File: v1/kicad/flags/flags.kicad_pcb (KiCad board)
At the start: 2 copper layers, 156.5 x 107.5 mm, 13 parts, among them J1 LNCPU_FLAGS_Connector, U1 74LS32, U10 74LS08, U11 74HC173, U12 74LS244, U2 74LS08, U3 74LS32, U4 74AHC04, U5 74LS32, U6 74LS157, U7 74LS157, U8 LNCPU Type B Connector, U9 74HC74

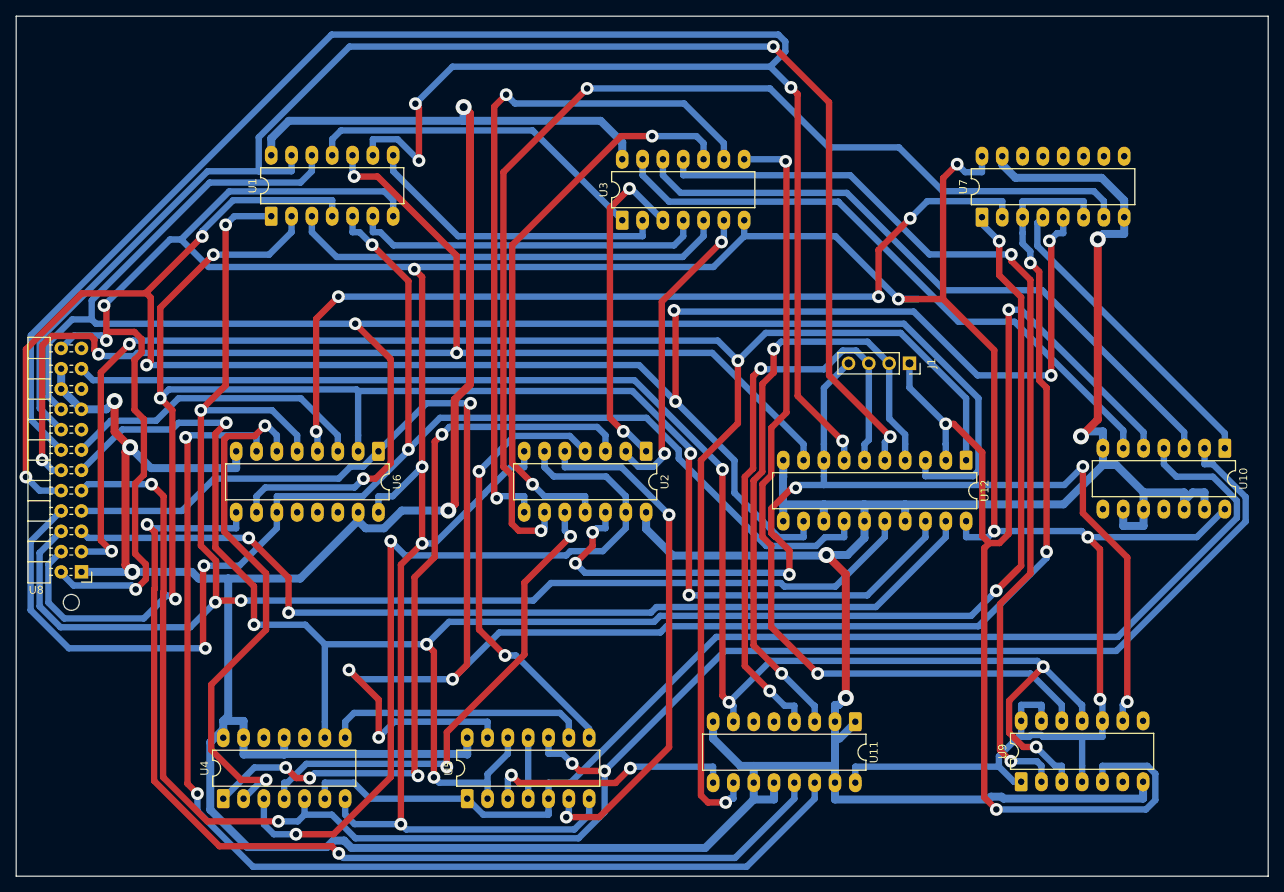
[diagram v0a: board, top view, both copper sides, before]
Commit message: partial on kicad flags
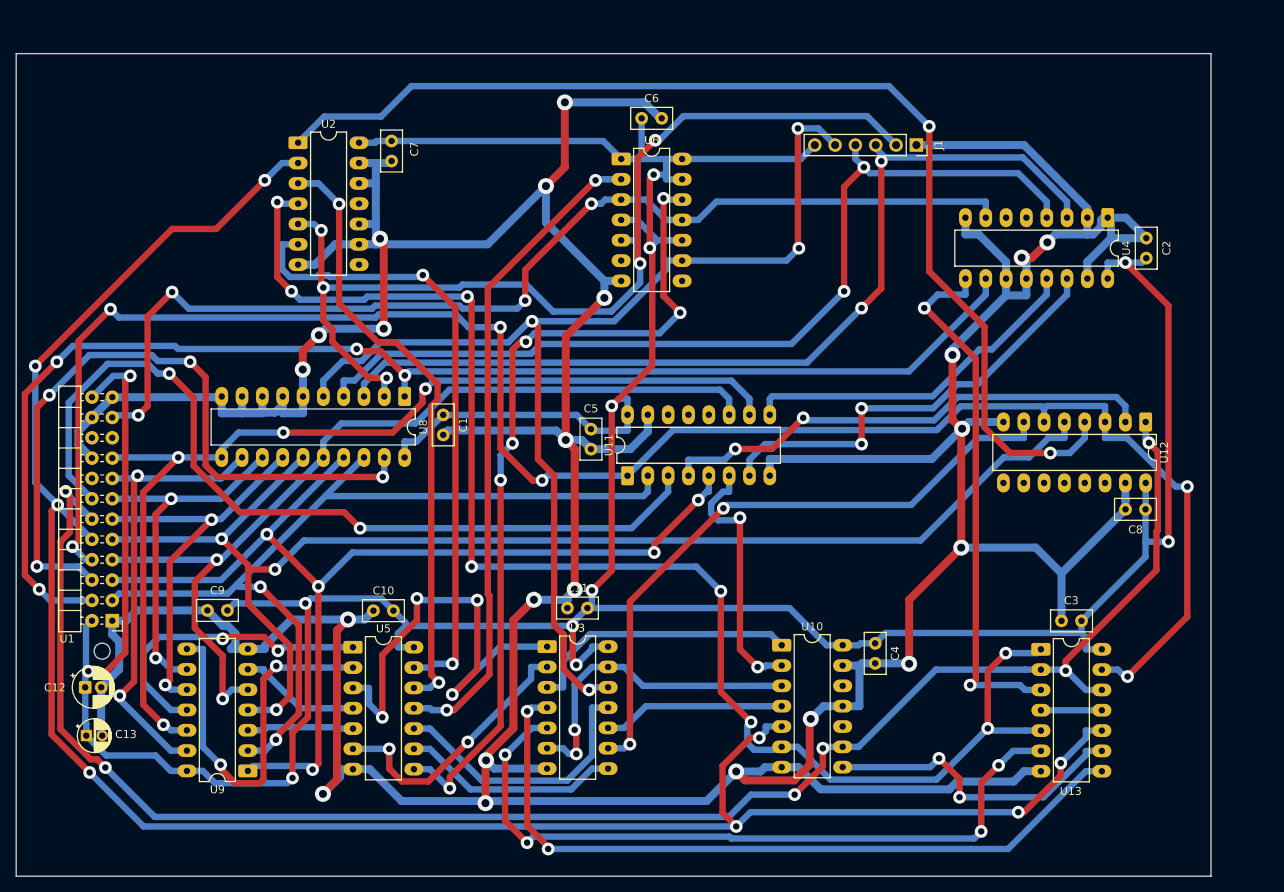
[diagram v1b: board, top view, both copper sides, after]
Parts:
- removed U7: 74LS157, Package_DIP:DIP-16_W7.62mm_LongPads
- added C1: 220n, Capacitor_THT:C_Disc_D5.0mm_W2.5mm_P2.50mm, F.Cu at (116.9, 72.3)
- added C10: 100n, Capacitor_THT:C_Disc_D5.0mm_W2.5mm_P2.50mm, F.Cu at (108.2, 96.8)
- added C11: 100n, Capacitor_THT:C_Disc_D5.0mm_W2.5mm_P2.50mm, F.Cu at (132.4, 96.5)
- added C12: C_Polarized, Capacitor_THT:CP_Radial_D5.0mm_P2.00mm, F.Cu at (72.1, 106.4)
- added C13: C_Polarized, lncpu:CP_Radial_D4.0mm_P2.00mm-Large-Holes, F.Cu at (72.3, 112.4)
- added C2: 220n, Capacitor_THT:C_Disc_D5.0mm_W2.5mm_P2.50mm, F.Cu at (204.8, 52.7)
- added C3: 100n, Capacitor_THT:C_Disc_D5.0mm_W2.5mm_P2.50mm, F.Cu at (196.7, 98.1)
- added C4: 100n, Capacitor_THT:C_Disc_D5.0mm_W2.5mm_P2.50mm, F.Cu at (170.9, 100.9)
- added C5: 100n, Capacitor_THT:C_Disc_D5.0mm_W2.5mm_P2.50mm, F.Cu at (135.3, 74.1)
- added C6: 100n, Capacitor_THT:C_Disc_D5.0mm_W2.5mm_P2.50mm, F.Cu at (141.7, 35.3)
- added C7: 100n, Capacitor_THT:C_Disc_D5.0mm_W2.5mm_P2.50mm, F.Cu at (110.4, 40.6)
- added C8: 100n, Capacitor_THT:C_Disc_D5.0mm_W2.5mm_P2.50mm, F.Cu at (202.2, 84.1)
- added C9: 100n, Capacitor_THT:C_Disc_D5.0mm_W2.5mm_P2.50mm, F.Cu at (87.4, 96.8)
- added U13: 74LS32, Package_DIP:DIP-14_W7.62mm_LongPads, F.Cu at (191.6, 101.6)
- J1: footprint Connector_PinSocket_2.54mm:PinSocket_1x04_P2.54mm_Vertical -> Connector_PinSocket_2.54mm:PinSocket_1x06_P2.54mm_Vertical
- U1: value 74LS32 -> LNCPU Type B Header; footprint Package_DIP:DIP-14_W7.62mm_LongPads -> lncpu:LNCPU_Type_B_Header
- U10: value 74LS08 -> 74LS04
- U11: value 74HC173 -> 74LS157
- U12: value 74LS244 -> 74LS157; footprint Package_DIP:DIP-20_W7.62mm_LongPads -> Package_DIP:DIP-16_W7.62mm_LongPads
- U3: value 74LS32 -> 74LS08
- U4: value 74AHC04 -> 74HCT173; footprint Package_DIP:DIP-14_W7.62mm_LongPads -> Package_DIP:DIP-16_W7.62mm_LongPads
- U6: value 74LS157 -> 74HCT74; footprint Package_DIP:DIP-16_W7.62mm_LongPads -> Package_DIP:DIP-14_W7.62mm_LongPads
- U8: value LNCPU Type B Connector -> 74HCT541; footprint lncpu:LNCPU_Type_B_Header -> Package_DIP:DIP-20_W7.62mm_LongPads
- U9: value 74HC74 -> 74LS32
- moved U4 132.3 mm to (199.9, 47.7), turned to -90 degrees
- moved U9 96.7 mm to (92.5, 116.8), turned to 180 degrees
- moved U10 60.6 mm to (159.2, 101.1), turned to 0 degrees
- moved U2 58.1 mm to (98.7, 38.3), turned to 0 degrees
- moved U1 54.3 mm to (75.5, 98.1), turned to 180 degrees
- moved U3 54.1 mm to (129.9, 101.3), turned to 0 degrees
- moved U6 47.5 mm to (139.1, 40.3), turned to 0 degrees
- moved U8 46.0 mm to (112.1, 70.0), turned to -90 degrees
- moved U11 41.9 mm to (139.9, 79.9), turned to 90 degrees
- moved J1 27.3 mm to (176.0, 38.6)
- moved U5 23.7 mm to (105.6, 101.4), turned to 0 degrees
- moved U12 22.9 mm to (204.7, 73.2)
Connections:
- J1 pad 1: Net-(J1-C) -> GND
- J1 pad 2: Net-(J1-Z) -> Net-(J1-C)
- J1 pad 3: Net-(J1-N) -> Net-(J1-Z)
- J1 pad 4: Net-(J1-I) -> Net-(J1-N)
- U1 pad 1: /FlagsCtrl/DBUS1 -> GND
- U1 pad 10: /FlagsCtrl/DBUS4 -> /FlagsCtrl/MODE_{1}
- U1 pad 11: Net-(U1-Pad11) -> /FlagsCtrl/DBUS4
- U1 pad 12: /FlagsCtrl/DBUS7 -> /FlagsCtrl/MODE_{2}
- U1 pad 13: /FlagsCtrl/DBUS6 -> /FlagsCtrl/DBUS5
- U1 pad 14: GND -> /FlagsCtrl/ALU_{Cin}
- U1 pad 2: /FlagsCtrl/DBUS0 -> VCC
- U1 pad 3: Net-(U1-Pad3) -> /FlagsCtrl/DBUS0
- U1 pad 4: /FlagsCtrl/DBUS3 -> Net-(U1-CTRL_{0})
- U1 pad 5: /FlagsCtrl/DBUS2 -> /FlagsCtrl/DBUS1
- U1 pad 6: Net-(U1-Pad6) -> Net-(U1-CTRL_{1})
- U1 pad 7: VCC -> /FlagsCtrl/DBUS2
- U1 pad 8: Net-(U1-Pad8) -> /FlagsCtrl/MODE_{0}
- U1 pad 9: /FlagsCtrl/DBUS5 -> /FlagsCtrl/DBUS3
- U10 pad 1: /FlagsCtrl/C_{val} -> Net-(U10-Pad1)
- U10 pad 10: GND -> unconnected-(U10-Pad10)
- U10 pad 11: unconnected-(U10-Pad11) -> GND
- U10 pad 12: GND -> unconnected-(U10-Pad12)
- U10 pad 2: /FlagsCtrl/MODE_{1} -> /FlagsCtrl/ALU_{Zin}
- U10 pad 3: Net-(U10-Pad3) -> /FlagsCtrl/~{I_{in}}
- U10 pad 4: /FlagsCtrl/~{MODE_{1}} -> /FlagsCtrl/I_{in}
- U10 pad 5: Net-(J1-C) -> /FlagsCtrl/MODE_{1}
- U10 pad 6: Net-(U10-Pad6) -> /FlagsCtrl/~{MODE_{1}}
- U10 pad 8: unconnected-(U10-Pad8) -> /FlagsCtrl/~{MODE_{2}}
- U10 pad 9: GND -> /FlagsCtrl/MODE_{2}
- U11 pad 1: GND -> /FlagsCtrl/MODE_{0}
- U11 pad 10: Net-(U11-E2) -> /FlagsCtrl/DBUS7
- U11 pad 11: GND -> /FlagsCtrl/DBUS2
- U11 pad 12: GND -> unconnected-(U11-Zd-Pad12)
- U11 pad 13: /FlagsCtrl/N_{val} -> unconnected-(U11-I1d-Pad13)
- U11 pad 14: /FlagsCtrl/Z_{val} -> unconnected-(U11-I0d-Pad14)
- U11 pad 2: GND -> /FlagsCtrl/DBUS0
- U11 pad 3: Net-(J1-Z) -> /FlagsCtrl/ALU_{Cin}
- U11 pad 4: Net-(J1-N) -> Net-(U11-Za)
- U11 pad 5: unconnected-(U11-Q2-Pad5) -> /FlagsCtrl/DBUS1
- U11 pad 6: unconnected-(U11-Q3-Pad6) -> /FlagsCtrl/ALU_{Zin}
- U11 pad 7: CLK -> /FlagsCtrl/Z_{val}
- U11 pad 9: /FlagsCtrl/~{CZ_{in}} -> /FlagsCtrl/N_{val}
- U12 pad 1: Net-(U11-E2) -> /FlagsCtrl/MODE_{2}
- U12 pad 10: GND -> unconnected-(U12-I1c-Pad10)
- U12 pad 11: GND -> unconnected-(U12-I0c-Pad11)
- U12 pad 12: /FlagsCtrl/DBUS3 -> unconnected-(U12-Zd-Pad12)
- U12 pad 13: GND -> unconnected-(U12-I1d-Pad13)
- U12 pad 14: /FlagsCtrl/DBUS2 -> unconnected-(U12-I0d-Pad14)
- U12 pad 16: /FlagsCtrl/DBUS1 -> VCC
- U12 pad 2: Net-(J1-C) -> Net-(U11-Za)
- U12 pad 3: /FlagsCtrl/DBUS7 -> /FlagsCtrl/MODE_{0}
- U12 pad 4: Net-(J1-Z) -> /FlagsCtrl/C_{val}
- U12 pad 5: /FlagsCtrl/DBUS6 -> /FlagsCtrl/DBUS3
- U12 pad 6: Net-(J1-N) -> /FlagsCtrl/MODE_{0}
- U12 pad 7: /FlagsCtrl/DBUS5 -> /FlagsCtrl/I_{val}
- U12 pad 8: Net-(J1-I) -> GND
- U12 pad 9: /FlagsCtrl/DBUS4 -> unconnected-(U12-Zc-Pad9)
- U2 pad 1: Net-(U2-Pad1) -> /FlagsCtrl/C_{val}
- U2 pad 10: /FlagsCtrl/I_{in} -> GND
- U2 pad 11: Net-(U2-Pad11) -> unconnected-(U2-Pad11)
- U2 pad 12: Net-(J1-I) -> GND
- U2 pad 13: /FlagsCtrl/~{I_{in}} -> GND
- U2 pad 14: GND -> VCC
- U2 pad 2: Net-(U2-Pad2) -> /FlagsCtrl/MODE_{1}
- U2 pad 4: Net-(U2-Pad4) -> /FlagsCtrl/~{MODE_{1}}
- U2 pad 5: Net-(U2-Pad5) -> Net-(J1-C)
- U2 pad 6: /FlagsCtrl/~{I_{in}} -> Net-(U2-Pad6)
- U2 pad 7: VCC -> GND
- U2 pad 8: Net-(U2-Pad8) -> unconnected-(U2-Pad8)
- U2 pad 9: /FlagsCtrl/I_{val} -> GND
- U3 pad 1: Net-(U1-Pad11) -> Net-(U3-Pad1)
- U3 pad 10: Net-(U2-Pad11) -> /FlagsCtrl/I_{in}
- U3 pad 11: Net-(U9A-D) -> Net-(U3-Pad11)
- U3 pad 12: Net-(U10-Pad3) -> Net-(J1-I)
- U3 pad 13: Net-(U10-Pad6) -> /FlagsCtrl/~{I_{in}}
- U3 pad 14: GND -> VCC
- U3 pad 2: Net-(U1-Pad8) -> Net-(U3-Pad2)
- U3 pad 3: Net-(U2-Pad1) -> Net-(U10-Pad1)
- U3 pad 4: Net-(U1-Pad6) -> Net-(U13-Pad8)
- U3 pad 5: Net-(U1-Pad3) -> Net-(U13-Pad6)
- U3 pad 6: Net-(U2-Pad2) -> /FlagsCtrl/~{I_{in}}
- U3 pad 7: VCC -> GND
- U3 pad 8: Net-(U9B-D) -> Net-(U3-Pad8)
- U3 pad 9: Net-(U2-Pad8) -> /FlagsCtrl/I_{val}
- U4 pad 1: Net-(U2-Pad3) -> GND
- U4 pad 10: unconnected-(U4-Pad10) -> Net-(U1-CTRL_{0})
- U4 pad 12: unconnected-(U4-Pad12) -> GND
- U4 pad 13: GND -> /FlagsCtrl/N_{val}
- U4 pad 14: GND -> /FlagsCtrl/Z_{val}
- U4 pad 2: /FlagsCtrl/ALU_{Zin} -> GND
- U4 pad 3: /FlagsCtrl/~{I_{in}} -> Net-(J1-Z)
- U4 pad 4: /FlagsCtrl/I_{in} -> Net-(J1-N)
- U4 pad 5: /FlagsCtrl/MODE_{1} -> unconnected-(U4-Q2-Pad5)
- U4 pad 6: /FlagsCtrl/~{MODE_{1}} -> unconnected-(U4-Q3-Pad6)
- U4 pad 7: VCC -> CLK
- U4 pad 8: /FlagsCtrl/~{MODE_{2}} -> GND
- U4 pad 9: /FlagsCtrl/MODE_{2} -> /FlagsCtrl/~{NZ_{in}}
- U5 pad 1: /FlagsCtrl/~{MODE_{1}} -> Net-(U5-Pad1)
- U5 pad 10: /FlagsCtrl/MODE_{1} -> Net-(U3-Pad11)
- U5 pad 11: Net-(U5-Pad11) -> Net-(U6A-D)
- U5 pad 12: /FlagsCtrl/MODE_{2} -> Net-(U2-Pad3)
- U5 pad 13: /FlagsCtrl/MODE_{0} -> Net-(U2-Pad6)
- U5 pad 14: GND -> VCC
- U5 pad 2: /FlagsCtrl/MODE_{2} -> Net-(U5-Pad2)
- U5 pad 3: /FlagsCtrl/~{CZ_{in}} -> Net-(U3-Pad1)
- U5 pad 4: Net-(U5-Pad11) -> Net-(U5-Pad4)
- U5 pad 5: /FlagsCtrl/~{MODE_{1}} -> Net-(U5-Pad5)
- U5 pad 6: Net-(U2-Pad5) -> Net-(U3-Pad2)
- U5 pad 7: VCC -> GND
- U5 pad 8: Net-(U2-Pad4) -> Net-(U6B-D)
- U5 pad 9: /FlagsCtrl/~{MODE_{2}} -> Net-(U3-Pad8)
- U6 pad 1: /FlagsCtrl/MODE_{0} -> VCC
- U6 pad 10: /FlagsCtrl/DBUS7 -> VCC
- U6 pad 11: /FlagsCtrl/DBUS2 -> CLK
- U6 pad 12: unconnected-(U6-Zd-Pad12) -> Net-(U6B-D)
- U6 pad 13: unconnected-(U6-I1d-Pad13) -> VCC
- U6 pad 14: unconnected-(U6-I0d-Pad14) -> VCC
- U6 pad 2: /FlagsCtrl/DBUS0 -> Net-(U6A-D)
- U6 pad 3: /FlagsCtrl/ALU_{Cin} -> CLK
- U6 pad 4: Net-(U6-Za) -> VCC
- U6 pad 5: /FlagsCtrl/DBUS1 -> Net-(J1-C)
- U6 pad 6: /FlagsCtrl/ALU_{Zin} -> unconnected-(U6A-~{Q}-Pad6)
- U6 pad 7: /FlagsCtrl/Z_{val} -> GND
- U6 pad 8: GND -> unconnected-(U6B-~{Q}-Pad8)
- U6 pad 9: /FlagsCtrl/N_{val} -> Net-(J1-I)
- U8 pad 1: GND -> Net-(U1-CTRL_{0})
- U8 pad 10: /FlagsCtrl/DBUS3 -> GND
- U8 pad 11: /FlagsCtrl/MODE_{2} -> /FlagsCtrl/DBUS7
- U8 pad 12: /FlagsCtrl/DBUS4 -> /FlagsCtrl/DBUS6
- U8 pad 13: /FlagsCtrl/ALU_{Cin} -> /FlagsCtrl/DBUS5
- U8 pad 14: /FlagsCtrl/DBUS5 -> /FlagsCtrl/DBUS4
- U8 pad 15: unconnected-(U8-CTRL_{6}-Pad15) -> /FlagsCtrl/DBUS3
- U8 pad 16: /FlagsCtrl/DBUS6 -> /FlagsCtrl/DBUS2
- U8 pad 17: GND -> /FlagsCtrl/DBUS1
- U8 pad 18: /FlagsCtrl/DBUS7 -> /FlagsCtrl/DBUS0
- U8 pad 19: unconnected-(U8-RST-Pad19) -> Net-(U1-CTRL_{1})
- U8 pad 2: VCC -> Net-(J1-C)
- U8 pad 20: GND -> VCC
- U8 pad 3: Net-(U11-E2) -> Net-(J1-Z)
- U8 pad 4: /FlagsCtrl/DBUS0 -> Net-(J1-N)
- U8 pad 5: Net-(U12-OEb) -> Net-(J1-I)
- U8 pad 6: /FlagsCtrl/DBUS1 -> GND
- U8 pad 7: /FlagsCtrl/MODE_{0} -> GND
- U8 pad 8: /FlagsCtrl/DBUS2 -> GND
- U8 pad 9: /FlagsCtrl/MODE_{1} -> GND
- U9 pad 1: VCC -> /FlagsCtrl/DBUS1
- U9 pad 10: VCC -> /FlagsCtrl/DBUS4
- U9 pad 11: CLK -> Net-(U5-Pad1)
- U9 pad 12: Net-(U9B-D) -> /FlagsCtrl/DBUS7
- U9 pad 13: VCC -> /FlagsCtrl/DBUS6
- U9 pad 2: Net-(U9A-D) -> /FlagsCtrl/DBUS0
- U9 pad 3: CLK -> Net-(U5-Pad5)
- U9 pad 4: VCC -> /FlagsCtrl/DBUS3
- U9 pad 5: Net-(J1-C) -> /FlagsCtrl/DBUS2
- U9 pad 6: unconnected-(U9A-~{Q}-Pad6) -> Net-(U5-Pad4)
- U9 pad 8: unconnected-(U9B-~{Q}-Pad8) -> Net-(U5-Pad2)
- U9 pad 9: Net-(J1-I) -> /FlagsCtrl/DBUS5
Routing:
- net Net-(U11-E2): track 213.0 -> 0.00 mm, vias 4 -> 0
- net /FlagsCtrl/DBUS5: track 245.5 -> 46.1 mm, vias 4 -> 2
- net Net-(U1-CTRL_{0}): track 0.00 -> 165.3 mm, vias 0 -> 4
- net /FlagsCtrl/DBUS6: track 185.9 -> 57.7 mm
- net Net-(U12-OEb): track 120.7 -> 0.00 mm, vias 2 -> 0
- net Net-(U9A-D): track 119.6 -> 0.00 mm, vias 2 -> 0
- net Net-(U6-Za): track 114.0 -> 0.00 mm, vias 4 -> 0
- net Net-(U9B-D): track 107.6 -> 0.00 mm, vias 2 -> 0
- net Net-(U6B-D): track 0.00 -> 104.2 mm, vias 0 -> 6
- net /FlagsCtrl/DBUS0: track 214.9 -> 110.8 mm, vias 5 -> 2
- net /FlagsCtrl/DBUS4: track 153.4 -> 50.6 mm, vias 4 -> 2
- net /FlagsCtrl/C_{val}: track 38.9 -> 141.0 mm, vias 0 -> 2
- net /FlagsCtrl/DBUS7: track 226.8 -> 127.5 mm, vias 2 -> 4
- net Net-(U13-Pad8): track 0.00 -> 94.2 mm, vias 0 -> 2
- net Net-(U13-Pad6): track 0.00 -> 91.6 mm, vias 0 -> 4
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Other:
- board size 156.5 x 107.5 mm -> 149.4 x 102.8 mm
